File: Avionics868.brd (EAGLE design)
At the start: 85.4 x 22.9 mm, 69 parts, among them SW1 B3U-1000P-2P-SMD, U1 ATSAMD21G18_QFN, U2 SPX3819M5-L-3-0, U3 MCP73831T-2ACI/OT, U4 MPU-9250, U5 SIM868, U6 BMP280, X1 JSTPH, X2 32.768, X3 ZX62-B-5PA, X4 104239-1430, X5 U-FL, X6 U-FL

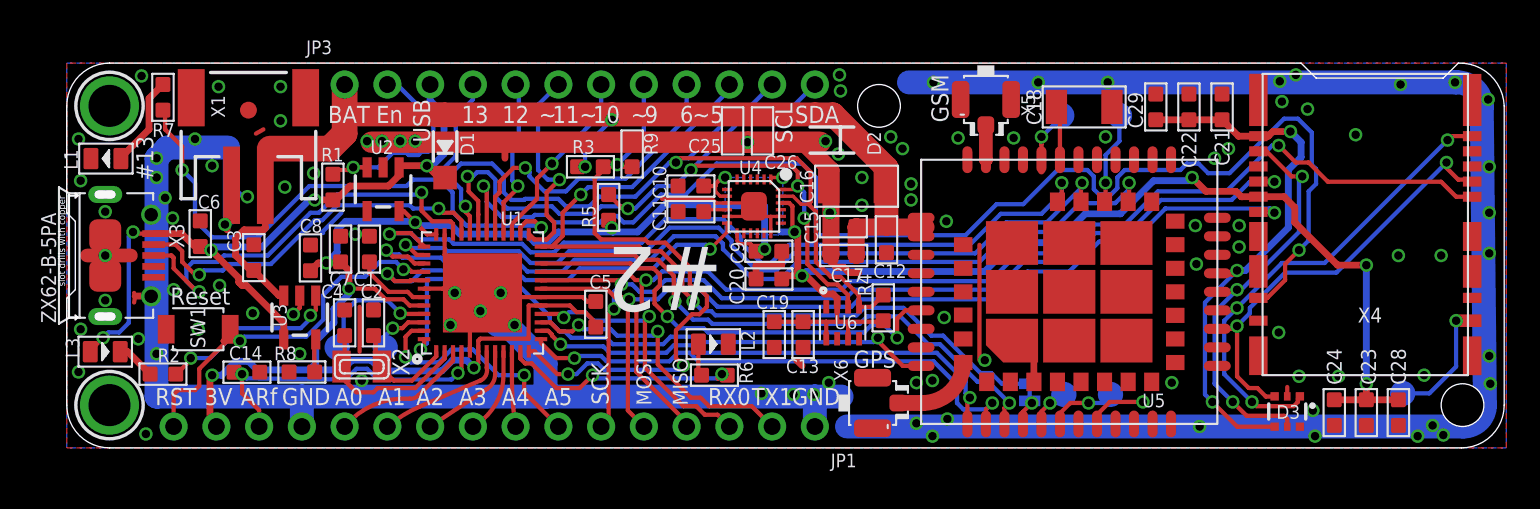
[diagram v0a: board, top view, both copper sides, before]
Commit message: Made it even a tiny bit shorter
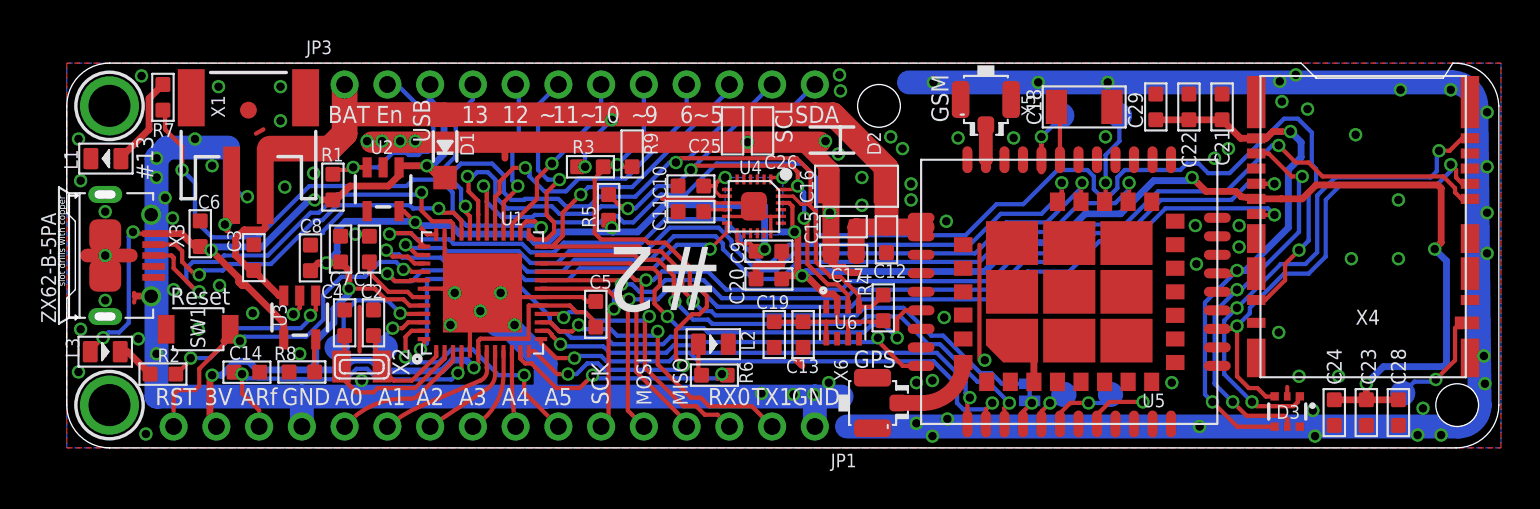
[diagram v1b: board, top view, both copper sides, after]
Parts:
- moved X4 0.18 mm to (77.0, 13.1)
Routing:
- net +3V: track 158.3 -> 170.0 mm
- net SIM_CLK: track 29.3 -> 31.8 mm
- net SIM_DATA: track 25.8 -> 27.9 mm
- net SD_DET: track 7.34 -> 6.68 mm
- net GND: track 260.5 -> 259.9 mm
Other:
- board size 85.4 x 22.9 mm -> 85.1 x 22.9 mm
